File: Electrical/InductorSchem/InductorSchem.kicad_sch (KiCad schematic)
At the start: 28 parts, among them J1 USB_C_Receptacle_USB2.0, J2 Battery, J3 Induction Charger, J4 VOut, J5 Breakout, SW1 SW_Push, SW10 SW_Push, SW11 SW_Push, SW12 SW_Push, SW2 SW_Push, SW3 SW_Push, SW4 SW_Push, SW5 SW_Push, SW6 SW_Push, SW7 SW_Push, SW8 SW_Push, SW9 SW_Push, U1 SeeeduinoXIAO, U2 InductorBMS, U3 MCP23018-E/SP

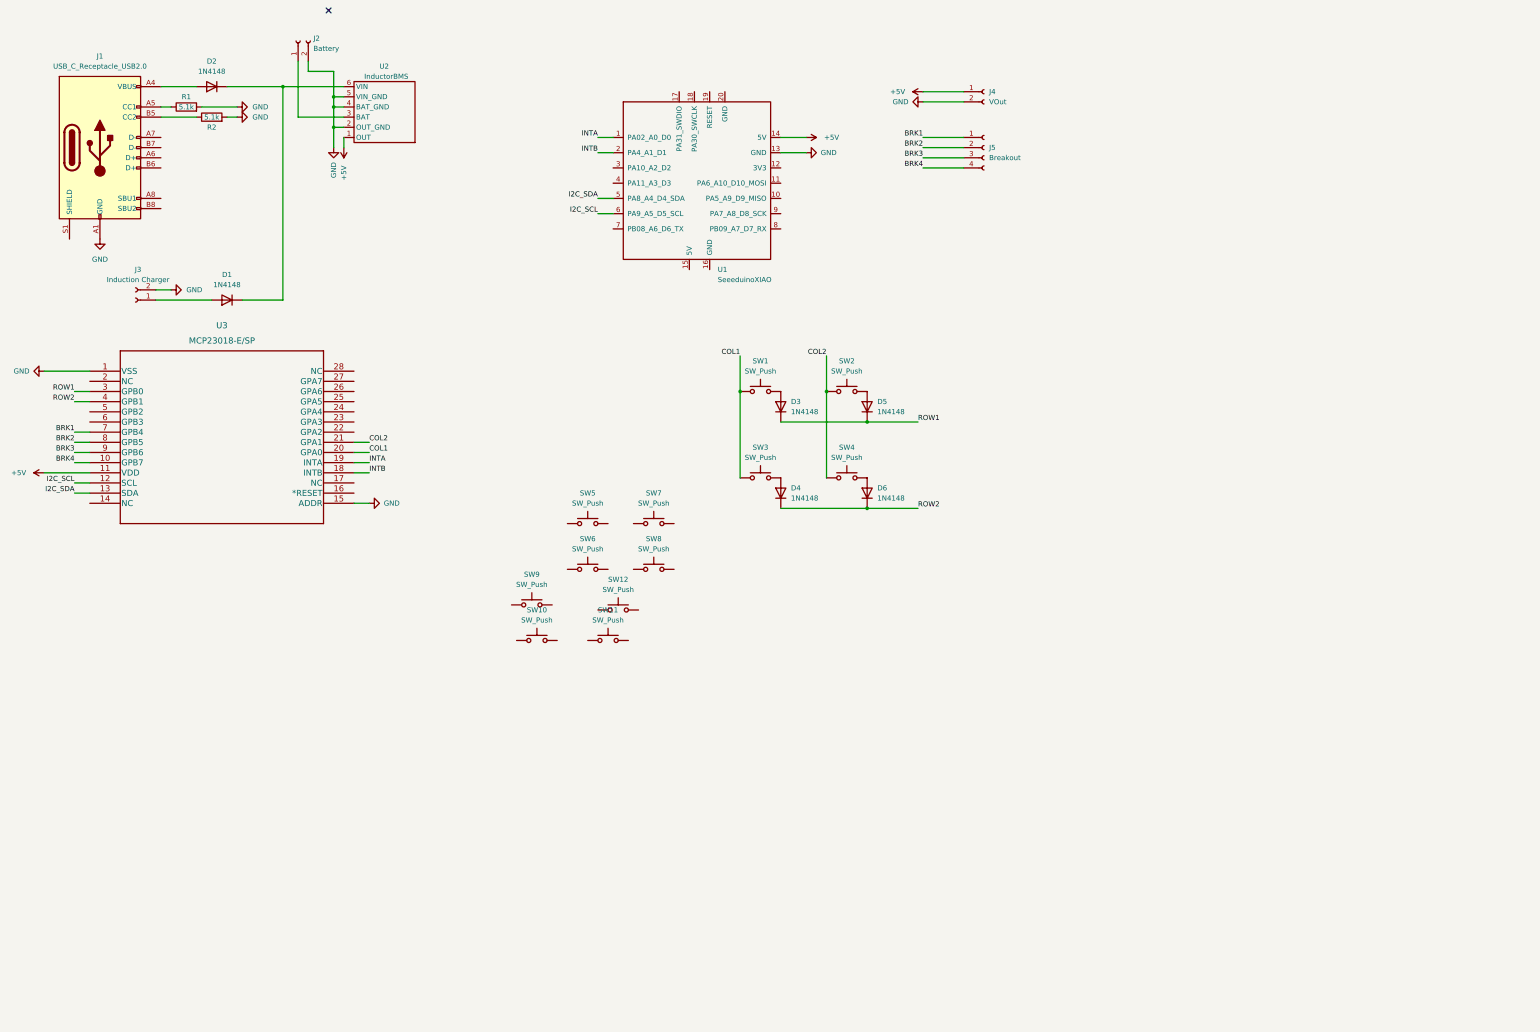
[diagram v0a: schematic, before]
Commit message: Full board
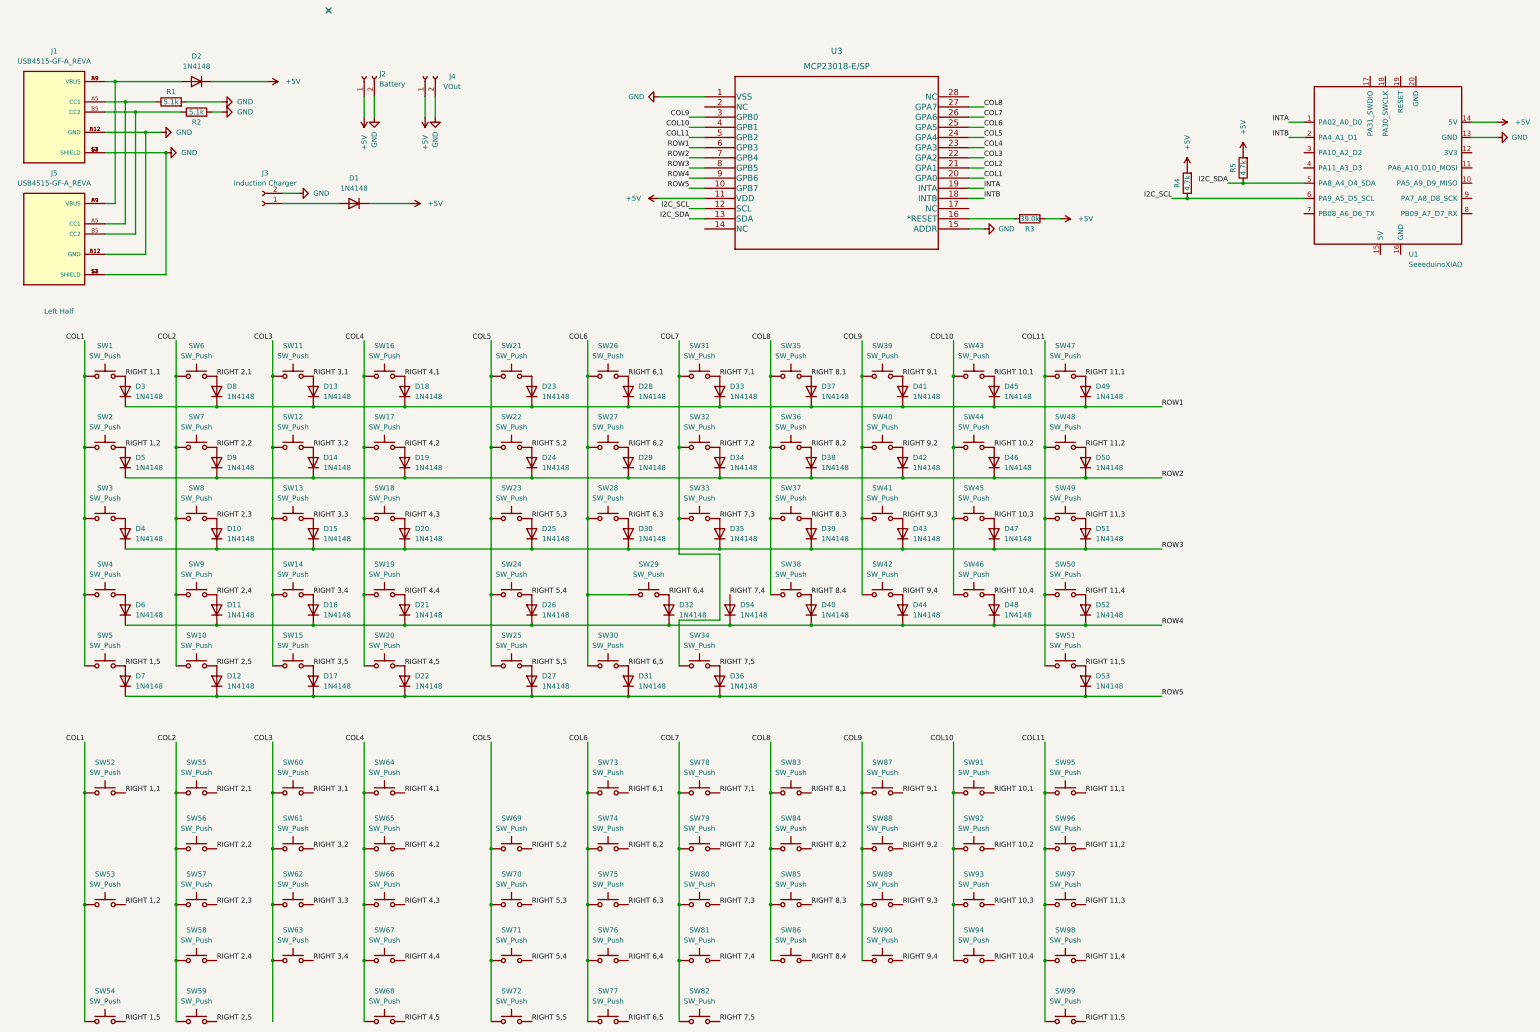
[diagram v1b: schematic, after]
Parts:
- removed J1: USB_C_Receptacle_USB2.0, Connector_USB:USB_C_Receptacle_GCT_USB4085, symbol Connector:USB_C_Receptacle_USB2.0
- removed J5: Breakout, Connector_Wire:SolderWire-0.5sqmm_1x04_P4.8mm_D0.9mm_OD2.3mm, symbol Connector:Conn_01x04_Female
- removed U2: InductorBMS, InductorProjFootprints:InductorBMS, symbol InductorProjLib:InductorBMS
- added D10, D11, D12, D13, D14, D15, D16, D17, D18, D19, D20, D21, D22, D23, D24, D25, D26, D27, D28, D29, D30, D31, D32, D33, D34, D35, D36, D37, D38, D39, D40, D41, D42, D43, D44, D45, D46, D47, D48, D49, D50, D51, D52, D53, D54, D7, D8, D9: 1N4148, Diode_THT:D_DO-35_SOD27_P7.62mm_Horizontal, symbol Diode:1N4148
- added J1, J5: USB4515-GF-A_REVA, GCT_USB4515-GF-A_REVA, symbol USB4515-GF-A_REVA:USB4515-GF-A_REVA
- added R3: 39.0k, Resistor_THT:R_Axial_DIN0207_L6.3mm_D2.5mm_P7.62mm_Horizontal, symbol Device:R
- added R4, R5: 4.7k, Resistor_THT:R_Axial_DIN0207_L6.3mm_D2.5mm_P7.62mm_Horizontal, symbol Device:R
- added SW13, SW14, SW15, SW16, SW17, SW18, SW19, SW20, SW21, SW22, SW23, SW24, SW25, SW26, SW27, SW28, SW30, SW31, SW32, SW33, SW34, SW35, SW36, SW37, SW38, SW39, SW40, SW41, SW42, SW43, SW44, SW45, SW46, SW47, SW48, SW49, SW50, SW51, SW52, SW55, SW56, SW57, SW58, SW59, SW60, SW61, SW62, SW63, SW64, SW65, SW66, SW67, SW69, SW70, SW71, SW72, SW74, SW75, SW76, SW77, SW78, SW79, SW80, SW81, SW82, SW83, SW84, SW85, SW86, SW87, SW88, SW89, SW90, SW91, SW92, SW93, SW94, SW95, SW96, SW97, SW98, SW99: SW_Push, Switch_Keyboard_Kailh:SW_Kailh_Choc_V1_1.00u, symbol Switch:SW_Push
- added SW29, SW68, SW73: SW_Push, Switch_Keyboard_Kailh:SW_Kailh_Choc_V1_2.00u_CUSTOMINDUCTOR, symbol Switch:SW_Push
- added SW53, SW54: SW_Push, Switch_Keyboard_Kailh:SW_Kailh_Choc_V1_2.00u_90deg, symbol Switch:SW_Push
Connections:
- net BRK1 is gone; now on net ROW2: U3.7 (GPB4)
- net +5V: now also D1.1 (K), D2.1 (K), J2.1 (Pin_1), R3.1, R4.2, R5.2
- net COL1: now also SW2.1, SW4.1, SW5.1, SW52.1, SW53.1, SW54.1
- net COL2: now also SW10.1, SW6.1, SW7.1, SW8.1, SW9.1, SW55.1, SW56.1, SW57.1, SW58.1, SW59.1; no longer SW2.1, SW4.1
- net GND: now also J1.A12 (GND), J1.B12 (GND), J1.S1 (SHIELD), J1.S2 (SHIELD), J1.S3 (SHIELD), J1.S4 (SHIELD), J5.A12 (GND), J5.B12 (GND), J5.S1 (SHIELD), J5.S2 (SHIELD), J5.S3 (SHIELD), J5.S4 (SHIELD)
- net I2C_SCL: now also R4.1
- net I2C_SDA: now also R5.1
- net ROW1: now also U3.6 (GPB3), D13.1 (K), D18.1 (K), D23.1 (K), D28.1 (K), D33.1 (K), D37.1 (K), D41.1 (K), D45.1 (K), D49.1 (K), D8.1 (K); no longer D5.1 (K), U3.3 (GPB0)
- net ROW2: now also D5.1 (K), D14.1 (K), D19.1 (K), D24.1 (K), D29.1 (K), D34.1 (K), D38.1 (K), D42.1 (K), D46.1 (K), D50.1 (K), D9.1 (K); no longer D4.1 (K), D6.1 (K), U3.4 (GPB1)
- net at U3.16 (*RESET): now also R3.2
- net COL3: now reaches U3.22 (GPA2)
- net COL3: now also SW11.1, SW12.1, SW13.1, SW14.1, SW15.1, SW60.1, SW61.1, SW62.1, SW63.1
- net COL4: now reaches U3.23 (GPA3)
- net COL4: now also SW16.1, SW17.1, SW18.1, SW19.1, SW20.1, SW64.1, SW65.1, SW66.1, SW67.1, SW68.1
- net COL5: now reaches U3.24 (GPA4)
- net COL5: now also SW21.1, SW22.1, SW23.1, SW24.1, SW25.1, SW69.1, SW70.1, SW71.1, SW72.1
- net COL6: now reaches U3.25 (GPA5)
- net COL6: now also SW26.1, SW27.1, SW28.1, SW29.1, SW30.1, SW73.1, SW74.1, SW75.1, SW76.1, SW77.1
- net COL7: now reaches U3.26 (GPA6)
- net COL7: now also SW31.1, SW32.1, SW33.1, SW34.1, SW78.1, SW79.1, SW80.1, SW81.1, SW82.1
- net COL8: now reaches U3.27 (GPA7)
- net COL8: now also SW35.1, SW36.1, SW37.1, SW38.1, SW83.1, SW84.1, SW85.1, SW86.1
- net COL11: now reaches U3.5 (GPB2)
- net COL11: now also SW47.1, SW48.1, SW49.1, SW50.1, SW51.1, SW95.1, SW96.1, SW97.1, SW98.1, SW99.1
- net at R1.1: now also J1.A5 (CC1), J5.A5 (CC1)
- net RIGHT 2,4: now reaches SW9.2
- net RIGHT 2,4: now also D11.2 (A), SW58.2
- net RIGHT 2,1: now reaches SW6.2
- net RIGHT 2,1: now also D8.2 (A), SW55.2
- net RIGHT 1,1: now reaches D3.2 (A), SW1.2
- net RIGHT 1,1: now also SW52.2
- net at D2.2 (A): now also J1.A9 (VBUS), J1.B9 (VBUS), J5.A9 (VBUS), J5.B9 (VBUS)
- net at R2.1: now also J1.B5 (CC2), J5.B5 (CC2)
- net RIGHT 3,2: now reaches SW12.2
- net RIGHT 3,2: now also D14.2 (A), SW61.2
- net RIGHT 1,2: now reaches D5.2 (A), SW2.2
- net RIGHT 1,2: now also SW53.2
- net RIGHT 2,2: now reaches SW7.2
- net RIGHT 2,2: now also D9.2 (A), SW56.2
- net RIGHT 3,1: now reaches SW11.2
- net RIGHT 3,1: now also D13.2 (A), SW60.2
- net RIGHT 2,5: now reaches SW10.2
- net RIGHT 2,5: now also D12.2 (A), SW59.2
- net RIGHT 1,5: now reaches SW5.2
- net RIGHT 1,5: now also D7.2 (A), SW54.2
- net RIGHT 2,3: now reaches SW8.2
- net RIGHT 2,3: now also D10.2 (A), SW57.2
- net BRK2 renamed ROW3
- net ROW3: now also D4.1 (K), D10.1 (K), D15.1 (K), D20.1 (K), D25.1 (K), D30.1 (K), D35.1 (K), D39.1 (K), D43.1 (K), D47.1 (K), D51.1 (K)
- net BRK3 renamed ROW4
- net ROW4: now also D6.1 (K), D11.1 (K), D16.1 (K), D21.1 (K), D26.1 (K), D32.1 (K), D40.1 (K), D44.1 (K), D48.1 (K), D52.1 (K), D54.1 (K)
- net BRK4 renamed ROW5
- net ROW5: now also D12.1 (K), D17.1 (K), D22.1 (K), D27.1 (K), D31.1 (K), D36.1 (K), D53.1 (K), D7.1 (K)
- new net: D23.2 (A), SW21.2
- new net COL10: SW43.1, SW44.1, SW45.1, SW46.1, SW91.1, SW92.1, SW93.1, SW94.1, U3.4 (GPB1)
- new net COL9: SW39.1, SW40.1, SW41.1, SW42.1, SW87.1, SW88.1, SW89.1, SW90.1, U3.3 (GPB0)
- new net RIGHT 10,1: D45.2 (A), SW43.2, SW91.2
- new net RIGHT 10,2: D46.2 (A), SW44.2, SW92.2
- new net RIGHT 10,3: D47.2 (A), SW45.2, SW93.2
- new net RIGHT 10,4: D48.2 (A), SW46.2, SW94.2
- new net RIGHT 11,1: D49.2 (A), SW47.2, SW95.2
- new net RIGHT 11,2: D50.2 (A), SW48.2, SW96.2
- new net RIGHT 11,3: D51.2 (A), SW49.2, SW97.2
- new net RIGHT 11,4: D52.2 (A), SW50.2, SW98.2
- new net RIGHT 11,5: D53.2 (A), SW51.2, SW99.2
- new net RIGHT 3,3: D15.2 (A), SW13.2, SW62.2
- new net RIGHT 3,4: D16.2 (A), SW14.2, SW63.2
- new net RIGHT 3,5: D17.2 (A), SW15.2
- new net RIGHT 4,1: D18.2 (A), SW16.2, SW64.2
- new net RIGHT 4,2: D19.2 (A), SW17.2, SW65.2
- new net RIGHT 4,3: D20.2 (A), SW18.2, SW66.2
- new net RIGHT 4,4: D21.2 (A), SW19.2, SW67.2
- new net RIGHT 4,5: D22.2 (A), SW20.2, SW68.2
- new net RIGHT 5,2: D24.2 (A), SW22.2, SW69.2
- new net RIGHT 5,3: D25.2 (A), SW23.2, SW70.2
- new net RIGHT 5,4: D26.2 (A), SW24.2, SW71.2
- new net RIGHT 5,5: D27.2 (A), SW25.2, SW72.2
- new net RIGHT 6,1: D28.2 (A), SW26.2, SW73.2
- new net RIGHT 6,2: D29.2 (A), SW27.2, SW74.2
- new net RIGHT 6,3: D30.2 (A), SW28.2, SW75.2
- new net RIGHT 6,4: D32.2 (A), SW29.2, SW76.2
- new net RIGHT 6,5: D31.2 (A), SW30.2, SW77.2
- new net RIGHT 7,1: D33.2 (A), SW31.2, SW78.2
- new net RIGHT 7,2: D34.2 (A), SW32.2, SW79.2
- new net RIGHT 7,3: D35.2 (A), SW33.2, SW80.2
- new net RIGHT 7,4: D54.2 (A), SW81.2
- new net RIGHT 7,5: D36.2 (A), SW34.2, SW82.2
- new net RIGHT 8,1: D37.2 (A), SW35.2, SW83.2
- new net RIGHT 8,2: D38.2 (A), SW36.2, SW84.2
- new net RIGHT 8,3: D39.2 (A), SW37.2, SW85.2
- new net RIGHT 8,4: D40.2 (A), SW38.2, SW86.2
- new net RIGHT 9,1: D41.2 (A), SW39.2, SW87.2
- new net RIGHT 9,2: D42.2 (A), SW40.2, SW88.2
- new net RIGHT 9,3: D43.2 (A), SW41.2, SW89.2
- new net RIGHT 9,4: D44.2 (A), SW42.2, SW90.2
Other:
- note added: "Left Half"
- moved on the sheet: D1, D2, D3, D4, D5, D6, J2, J3, J4, R1, R2, SW1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
